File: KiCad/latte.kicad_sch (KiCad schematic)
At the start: 152 parts, among them J1 Conn_01x04, U1 ATmega32U4-AU, Y1 Resonator_Small

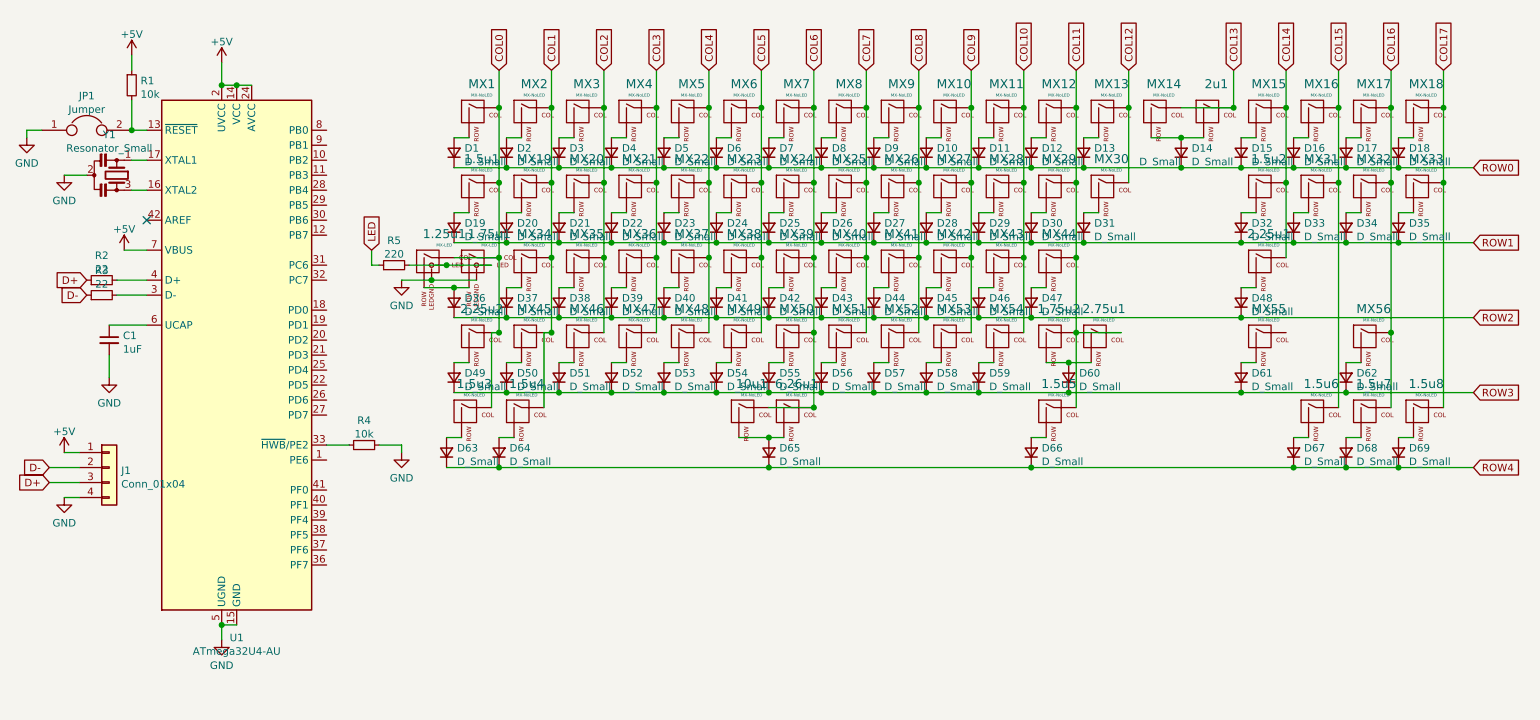
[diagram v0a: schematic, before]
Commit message: placed components
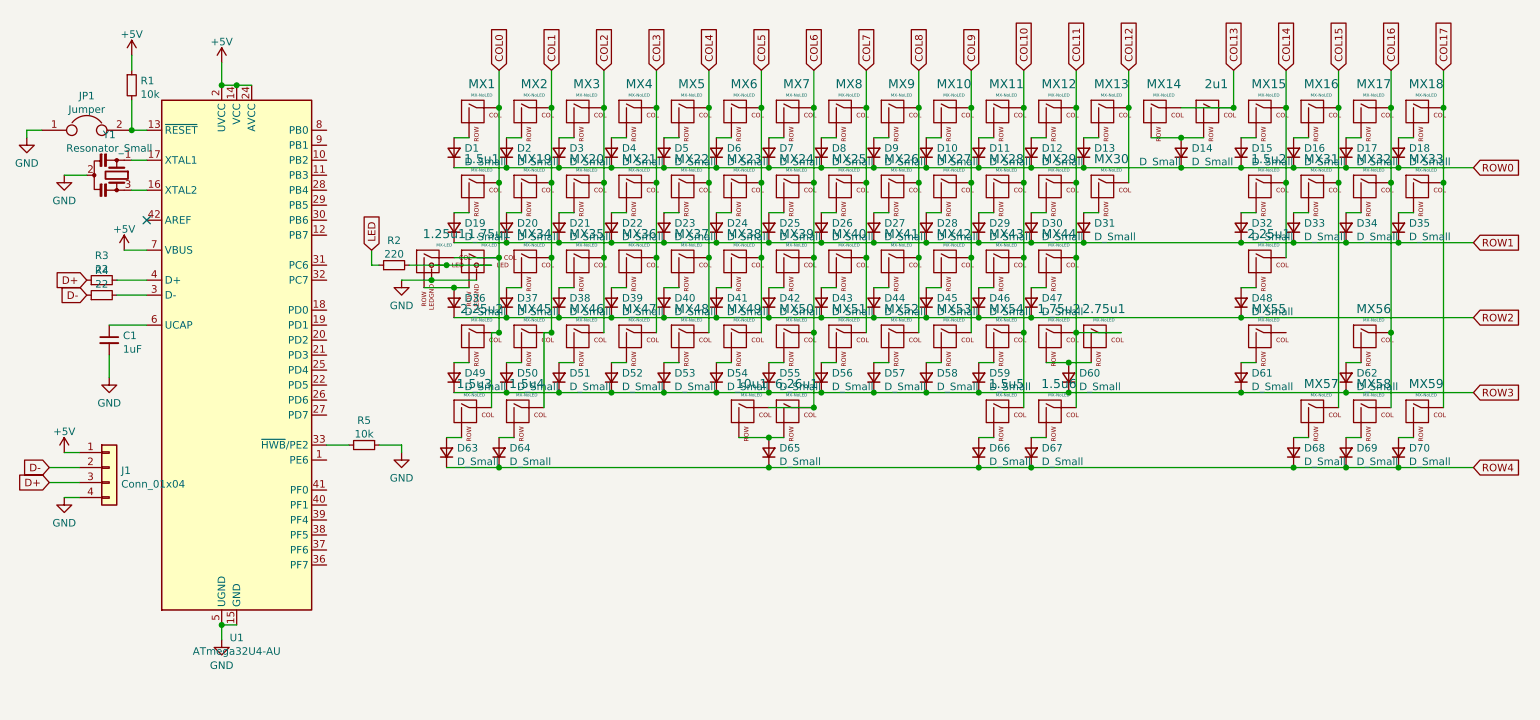
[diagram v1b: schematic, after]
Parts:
- removed 1.5u6, 1.5u7, 1.5u8: MX-NoLED, MX_Only:MXOnly-1.5U-NoLED, symbol MX_Alps_Hybrid:MX-NoLED
- added 1.5u5: MX-NoLED, MX_Only:MXOnly-1.5U-NoLED, symbol MX_Alps_Hybrid:MX-NoLED
- added D66: D_Small, Footprints:D_SOD-123-Pretty, symbol Device:D_Small
- added MX57, MX58, MX59: MX-NoLED, MX_Only:MXOnly-1U-NoLED, symbol MX_Alps_Hybrid:MX-NoLED
- 10u1: footprint Footprints:MX-10U -> Footprints:MXOnly-10U-NoLED
- R2: renamed from R5; footprint (none) -> Footprints:R_0805_2012Metric
- renumbered 1.5u5 to 1.5u6, D66 to D67, D67 to D68, D68 to D69, D69 to D70, R2 to R3, R3 to R4, R4 to R5
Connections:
- net COL10: now also 1.5u5.1 (COL)
- net COL15: now also MX57.1 (COL)
- net COL16: now also MX58.1 (COL)
- net COL17: now also MX59.1 (COL)
- net ROW4: now also D66.1 (K)
- net at D69.2 (A): now also MX58.2 (ROW)
- net at D70.2 (A): now also MX59.2 (ROW)
- net at D68.2 (A): now also MX57.2 (ROW)
- new net: 1.5u5.2 (ROW), D66.2 (A)

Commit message: honestly bro i forget what i did here
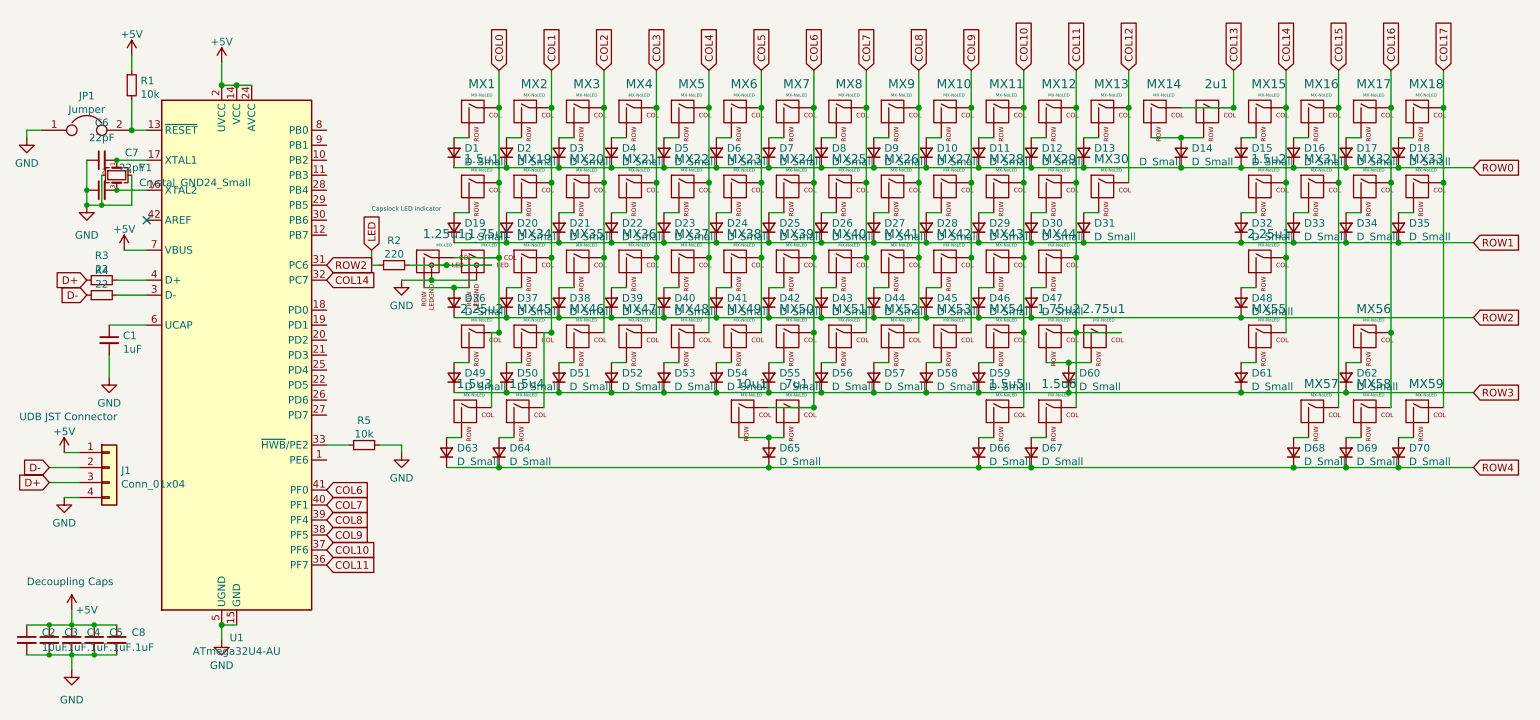
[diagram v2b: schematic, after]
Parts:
- removed Y1: Resonator_Small, Footprints:Resonator_SMD_muRata_CSTxExxV-3Pin_3.0x1.1mm, symbol Device:Resonator_Small
- added C2: 10uF, keeb:C_0805_2012Metric, symbol Device:C_Small
- added C3, C4, C5, C8: .1uF, keeb:C_0805_2012Metric, symbol Device:C_Small
- added C6, C7: 22pF, keeb:C_0805_2012Metric, symbol Device:C_Small
- added Y1: Crystal_GND24_Small, keeb:Crystal_SMD_3225-4Pin_3.2x2.5mm_HandSoldering, symbol Device:Crystal_GND24_Small
- 10u1: footprint Footprints:MXOnly-10U-NoLED -> keeb:MX-10U-NoSwitch-ReversedStabilizers
- 7u1: renamed from 6.26u1; footprint MX_Only:MXOnly-6.25U-NoLED -> MX_Only:MXOnly-7U-ReversedStabilizers-NoLED
- C1: footprint Footprints:C_0805_2012Metric -> keeb:C_0805_2012Metric
- D1, D10, D11, D12, D13, D14, D15, D16, D17, D18, D19, D2, D20, D21, D22, D23, D24, D25, D26, D27, D28, D29, D3, D30, D31, D32, D33, D34, D35, D36, D37, D38, D39, D4, D40, D41, D42, D43, D44, D45, D46, D47, D48, D49, D5, D50, D51, D52, D53, D54, D55, D56, D57, D58, D59, D6, D60, D61, D62, D63, D64, D65, D66, D67, D68, D69, D7, D70, D8, D9: footprint Footprints:D_SOD-123-Pretty -> keeb:D_SOD-123-Pretty
- J1: footprint Footprints:JST-SR-4 -> keeb:JST-SR-4
- JP1: footprint Footprints:ResetJumper -> keeb:ResetJumper
- R1, R2, R3, R4, R5: footprint Footprints:R_0805_2012Metric -> keeb:R_0805_2012Metric
- U1: footprint Package_QFP:TQFP-44_10x10mm_P0.8mm -> keeb:QFN_TQFP-44_Combined
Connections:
- net +5V: now also C2.1, C3.1, C4.1, C5.1, C8.1
- net COL10: now also U1.37 (PF6)
- net COL11: now also U1.36 (PF7)
- net COL14: now also MX55.1 (COL), U1.32 (PC7)
- net COL6: now also U1.41 (PF0)
- net COL7: now also U1.40 (PF1)
- net COL8: now also U1.39 (PF4)
- net COL9: now also U1.38 (PF5)
- net GND: now also C2.2, C3.2, C4.2, C5.2, C6.1, C7.1, C8.2, Y1.2, Y1.4
- net ROW2: now also U1.31 (PC6)
- net at U1.17 (XTAL1): now also C6.2, Y1.1
- net at U1.16 (XTAL2): now also C7.2, Y1.3
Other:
- note added: "Capslock LED indicator"
- note added: "Decoupling Caps"
- note added: "UDB JST Connector"

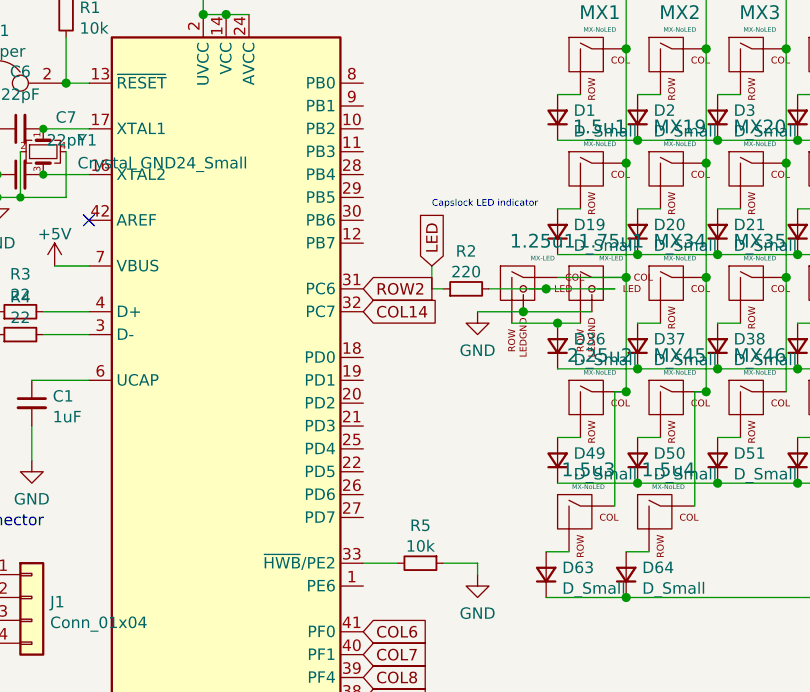
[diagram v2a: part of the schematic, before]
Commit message: finish v1
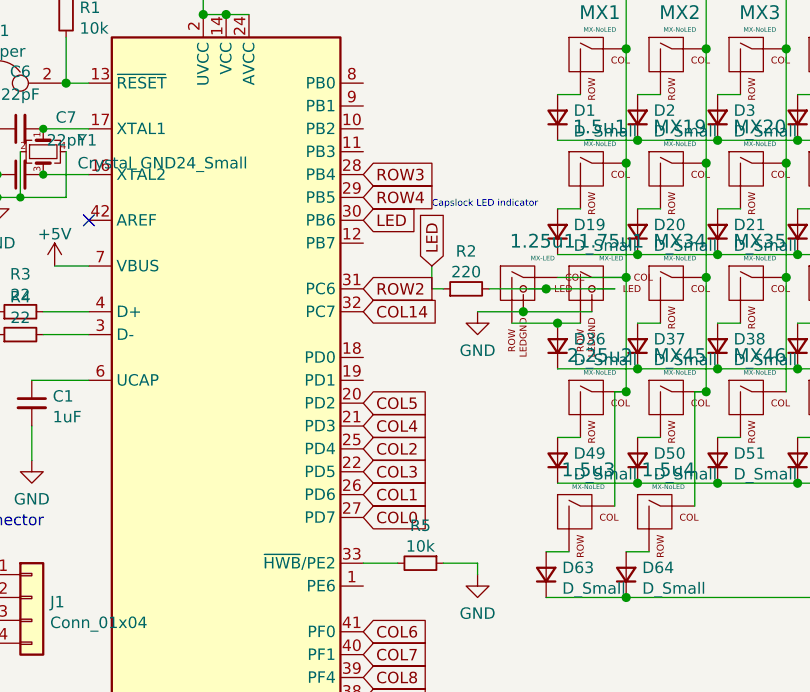
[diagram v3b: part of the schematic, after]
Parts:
- 10u1: footprint keeb:MX-10U-NoSwitch-ReversedStabilizers -> keeb:MX-8U-NoSwitch
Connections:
- net COL0: now also U1.27 (PD7)
- net COL1: now also U1.26 (PD6)
- net COL2: now also U1.25 (PD4)
- net COL3: now also U1.22 (PD5)
- net COL4: now also U1.21 (PD3)
- net COL5: now also U1.20 (PD2)
- net LED: now also U1.30 (PB6)
- net ROW3: now also U1.28 (PB4)
- net ROW4: now also U1.29 (PB5)
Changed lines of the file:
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@@
     )
   )
+  (global_label "ROW3" (shape input) (at 66.04 40.64 0) (fields_autoplaced)
+    (effects (font (size 1.27 1.27)) (justify left))
+    (property "Intersheet References" "${INTERSHEET_REFS}" (id 0) (at 73.7145 40.5606 0)
+      (effects (font (size 1.27 1.27)) (justify left) hide)
+    )
+  )
+  (global_label "ROW4" (shape input) (at 66.04 43.18 0) (fields_autoplaced)
+    (effects (font (size 1.27 1.27)) (justify left))
+    (property "Intersheet References" "${INTERSHEET_REFS}" (id 0) (at 73.7145 43.1006 0)
+      (effects (font (size 1.27 1.27)) (justify left) hide)
+    )
+  )
+  (global_label "LED" (shape input) (at 66.04 45.72 0) (fields_autoplaced)
+    (effects (font (size 1.27 1.27)) (justify left))
+    (property "Intersheet References" "${INTERSHEET_REFS}" (id 0) (at 71.9002 45.6406 0)
+      (effects (font (size 1.27 1.27)) (justify left) hide)
+    )
+  )
   (global_label "ROW2" (shape input) (at 66.04 53.34 0) (fields_autoplaced)
     (effects (font (size 1.27 1.27)) (justify left))
@@
     )
   )
+  (global_label "COL5" (shape input) (at 66.04 66.04 0) (fields_autoplaced)
+    (effects (font (size 1.27 1.27)) (justify left))
+    (property "Intersheet References" "${INTERSHEET_REFS}" (id 0) (at 73.2912 65.9606 0)
+      (effects (font (size 1.27 1.27)) (justify left) hide)
+    )
+  )
+  (global_label "COL4" (shape input) (at 66.04 68.58 0) (fields_autoplaced)
+    (effects (font (size 1.27 1.27)) (justify left))
+    (property "Intersheet References" "${INTERSHEET_REFS}" (id 0) (at 73.2912 68.5006 0)
+      (effects (font (size 1.27 1.27)) (justify left) hide)
+    )
+  )
+  (global_label "COL2" (shape input) (at 66.04 71.12 0) (fields_autoplaced)
+    (effects (font (size 1.27 1.27)) (justify left))
+    (property "Intersheet References" "${INTERSHEET_REFS}" (id 0) (at 73.2912 71.0406 0)
+      (effects (font (size 1.27 1.27)) (justify left) hide)
+    )
+  )
+  (global_label "COL3" (shape input) (at 66.04 73.66 0) (fields_autoplaced)
+    (effects (font (size 1.27 1.27)) (justify left))
+    (property "Intersheet References" "${INTERSHEET_REFS}" (id 0) (at 73.2912 73.5806 0)
+      (effects (font (size 1.27 1.27)) (justify left) hide)
+    )
+  )
+  (global_label "COL1" (shape input) (at 66.04 76.2 0) (fields_autoplaced)
+    (effects (font (size 1.27 1.27)) (justify left))
+    (property "Intersheet References" "${INTERSHEET_REFS}" (id 0) (at 73.2912 76.1206 0)
+      (effects (font (size 1.27 1.27)) (justify left) hide)
+    )
+  )
+  (global_label "COL0" (shape input) (at 66.04 78.74 0) (fields_autoplaced)
+    (effects (font (size 1.27 1.27)) (justify left))
+    (property "Intersheet References" "${INTERSHEET_REFS}" (id 0) (at 73.2912 78.6606 0)
+      (effects (font (size 1.27 1.27)) (justify left) hide)
+    )
+  )
   (global_label "COL6" (shape input) (at 66.04 91.44 0) (fields_autoplaced)
     (effects (font (size 1.27 1.27)) (justify left))
@@
       (effects (font (size 0.508 0.508)))
     )
-    (property "Footprint" "keeb:MX-10U-NoSwitch-ReversedStabilizers" (id 2) (at 121.285 79.375 0)
+    (property "Footprint" "keeb:MX-8U-NoSwitch" (id 2) (at 121.285 79.375 0)
       (effects (font (size 1.524 1.524)) hide)
     )
@@
     )
     (path "/c2b2f65c-9c8b-46cc-a72f-8e93c0aedb5b"
-      (reference "10u1") (unit 1) (value "MX-NoLED") (footprint "keeb:MX-10U-NoSwitch-ReversedStabilizers")
+      (reference "10u1") (unit 1) (value "MX-NoLED") (footprint "keeb:MX-8U-NoSwitch")
     )
     (path "/a4c4f2c4-03a3-4a13-80d7-2a427aa655ac"
